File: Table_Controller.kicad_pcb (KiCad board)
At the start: 2 copper layers, 141.6 x 116.3 mm, 98 parts, among them J10 1050171001 Micro Type B, J11 HX JN1.27-2x5 WZ H4.9, J12 Conn_01x04_Pin, J13 Conn_01x14_Pin, J14 2.54 mm header, J15 2.54 mm header, U10 STM32G431K8Tx, U11 LMR380x0, U12 VNH7070, Y10 20 MHz

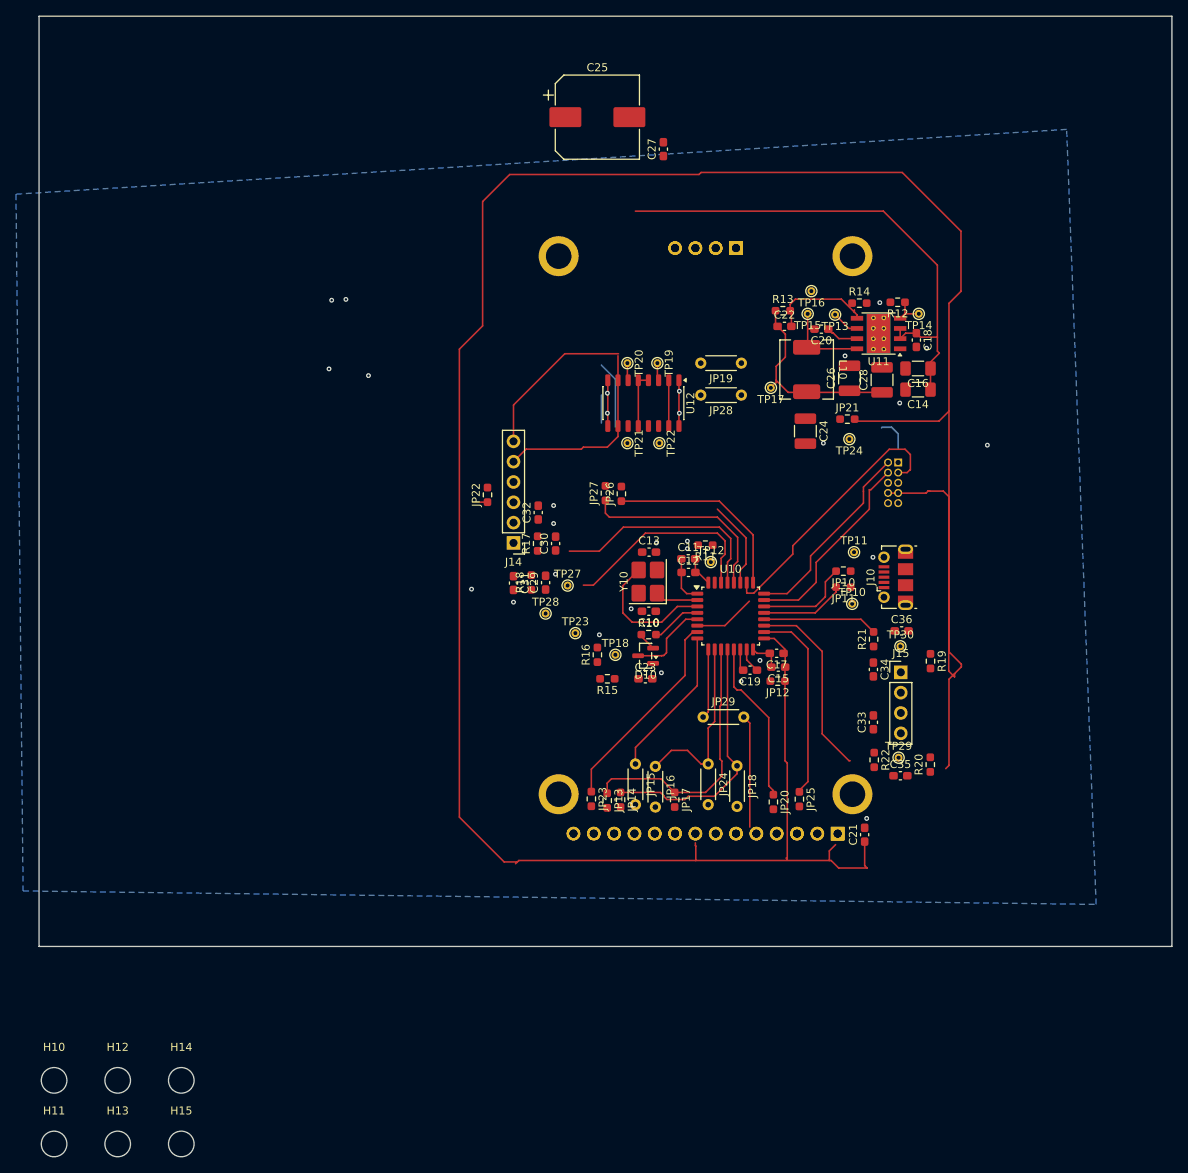
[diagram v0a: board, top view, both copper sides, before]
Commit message: Placement proposal 90%
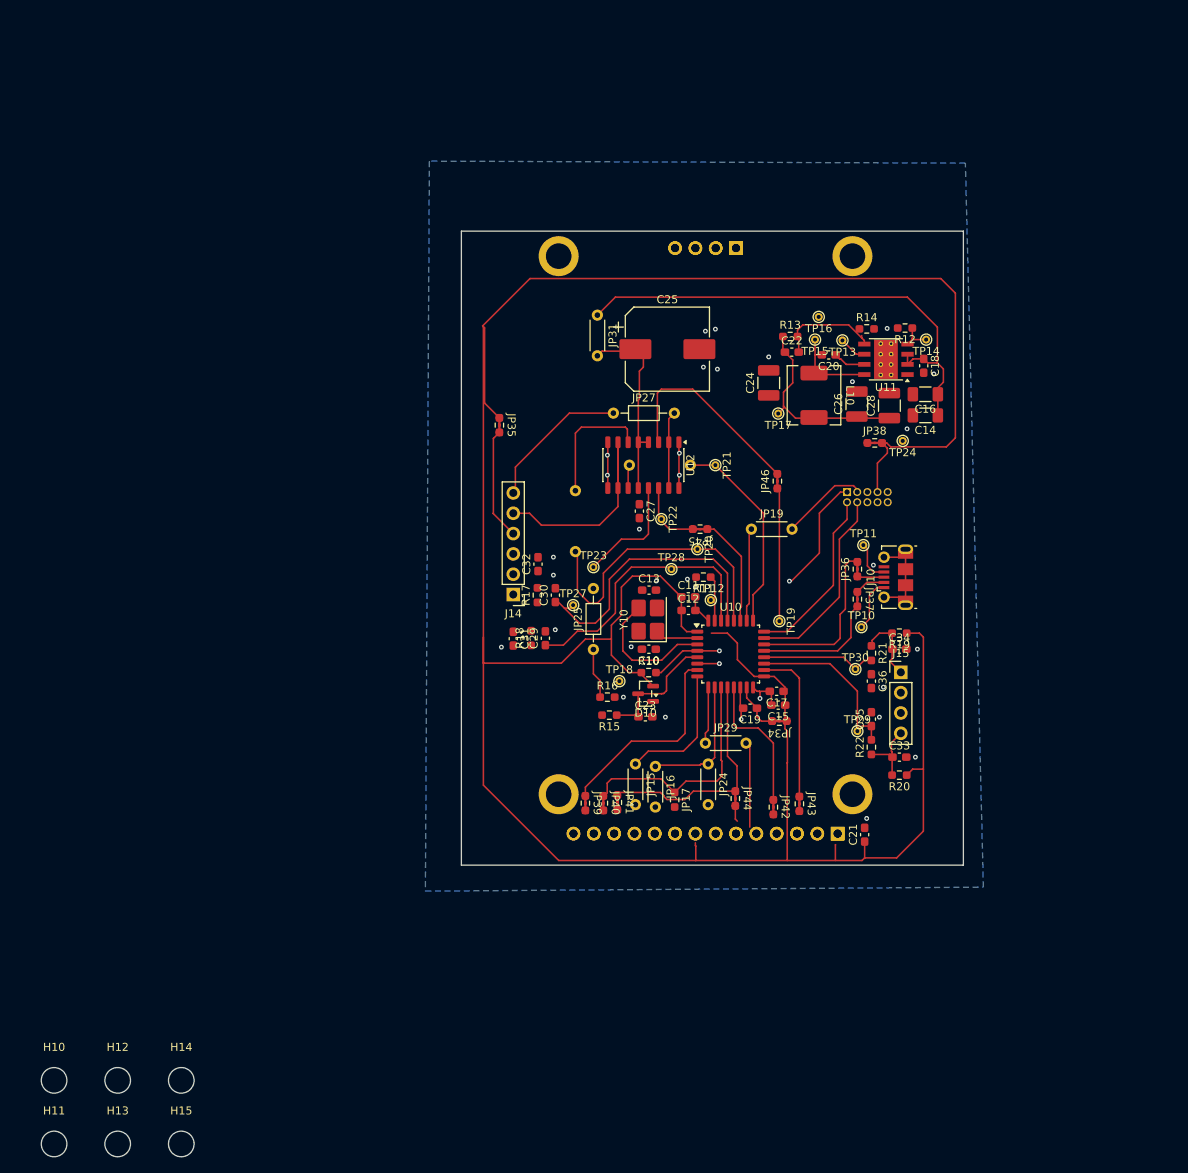
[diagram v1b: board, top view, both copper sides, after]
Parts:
- removed JP10, JP11, JP12, JP13, JP14, JP20, JP21, JP22, JP23: 0R, Resistor_SMD:R_0603_1608Metric_Pad0.98x0.95mm_HandSolder
- removed JP18, JP28: 0R, Resistor_THT:R_Axial_DIN0204_L3.6mm_D1.6mm_P5.08mm_Horizontal
- added JP31: 0R, Resistor_THT:R_Axial_DIN0204_L3.6mm_D1.6mm_P5.08mm_Horizontal, F.Cu at (95.8, 77.5)
- added JP32: 0R, Resistor_THT:R_Axial_DIN0204_L3.6mm_D1.6mm_P7.62mm_Horizontal, B.Cu at (99.8, 96.2)
- added JP34: 0R, Personal:Jumper_0603, F.Cu at (118.5, 128.2)
- added JP35: 0R, Personal:Jumper_0603, F.Cu at (83.5, 91.2)
- added JP36: 0R, Personal:Jumper_0603, F.Cu at (128.2, 109.2)
- added JP37: 0R, Personal:Jumper_0603, F.Cu at (128.2, 113.0)
- added JP38: 0R, Personal:Jumper_0603, F.Cu at (130.4, 93.5)
- added JP39: 0R, Personal:Jumper_0603, F.Cu at (94.2, 138.5)
- added JP40: 0R, Personal:Jumper_0603, F.Cu at (96.5, 138.5)
- added JP41: 0R, Personal:Jumper_0603, F.Cu at (98.2, 138.4)
- added JP42: 0R, Personal:Jumper_0603, F.Cu at (117.8, 139.0)
- added JP43: 0R, Personal:Jumper_0603, F.Cu at (121.0, 138.6)
- added JP44: 0R, Personal:Jumper_0603, F.Cu at (113.0, 137.9)
- added JP45: 0R, Personal:Jumper_0603, F.Cu at (108.6, 104.2)
- added JP46: 0R, Personal:Jumper_0603, F.Cu at (118.2, 98.2)
- JP25, JP27: footprint Resistor_SMD:R_0603_1608Metric_Pad0.98x0.95mm_HandSolder -> Resistor_THT:R_Axial_DIN0204_L3.6mm_D1.6mm_P7.62mm_Horizontal
- JP26: footprint Resistor_SMD:R_0603_1608Metric_Pad0.98x0.95mm_HandSolder -> Resistor_THT:R_Axial_DIN0204_L3.6mm_D1.6mm_P7.62mm_Horizontal; moved to B.Cu
- moved C27 45.3 mm to (101.0, 102.0), turned to -90 degrees
- moved TP19 35.7 mm to (118.5, 115.8)
- moved JP25 31.8 mm to (95.2, 119.3), turned to 90 degrees
- moved C25 30.3 mm to (104.5, 81.8)
- moved TP20 24.8 mm to (108.2, 106.8)
- moved JP19 20.8 mm to (115.0, 104.2), turned to 0 degrees
- moved TP28 16.7 mm to (105.0, 109.2)
- moved TP21 11.3 mm to (110.5, 96.2)
- moved JP27 10.0 mm to (97.8, 89.8), turned to 0 degrees
- moved TP22 9.50 mm to (103.8, 103.0)
- moved TP23 8.55 mm to (95.2, 109.0)
- moved C35 7.95 mm to (130.0, 128.0), turned to 90 degrees
- moved U12 7.75 mm to (101.5, 96.2)
- moved C24 7.57 mm to (117.2, 86.0), turned to 90 degrees
- moved C36 7.33 mm to (130.0, 123.2), turned to -90 degrees
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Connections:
- net Net-(U10-PF0) renamed /XIN
- net Net-(U10-PF1) renamed /XOUT
- C25 pad 1: /S19V5 -> Net-(C25-Pad1)
- C27 pad 1: /S19V5 -> Net-(C25-Pad1)
- J11 pad 3: /SWO -> Net-(J11-Pin_3)
- JP19 pad 1: /SEL0 -> /SWO
- JP19 pad 2: Net-(U12-SEL0) -> Net-(J11-Pin_3)
- JP25 pad 1: /DISP_CS -> Net-(JP25-Pad1)
- JP25 pad 2: Net-(J13-Pin_3) -> Net-(U12-CS)
- JP26 pad 1: /INa -> Net-(U12-INb)
- JP26 pad 2: Net-(U12-INa) -> /INb
- JP27 pad 1: /INb -> /OUTa
- JP27 pad 2: Net-(U12-INb) -> Net-(JP27-Pad2)
- R15 pad 2: Net-(U12-CS) -> Net-(JP25-Pad1)
- R16 pad 1: Net-(U12-CS) -> Net-(JP25-Pad1)
- TP19 pad 1: Net-(U12-INa) -> /INa
- TP20 pad 1: Net-(U12-INb) -> /INb
- TP21 pad 1: Net-(U12-PWM) -> /PWM
- U10 pad 25: /INa -> /PWM
- U10 pad 27: /PWM -> /SEL0
- U10 pad 6: /SEL0 -> /INa
- U12 pad 12: /S19V5 -> Net-(C25-Pad1)
- U12 pad 15: /OUTa -> Net-(JP27-Pad2)
- U12 pad 2: /OUTa -> Net-(JP27-Pad2)
- U12 pad 4: /S19V5 -> Net-(C25-Pad1)
- U12 pad 5: /S19V5 -> Net-(C25-Pad1)
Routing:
- net /NRST: track 10.6 -> 36.2 mm, vias 0 -> 2
- net Net-(C25-Pad1): track 0.00 -> 24.4 mm
- net /SWO: track 33.7 -> 11.7 mm
- net Net-(U12-INa): track 10.7 -> 25.8 mm
- net /PWM: track 11.0 -> 25.6 mm
- net Net-(U12-CS): track 0.00 -> 14.4 mm
- net Net-(J14-Pin_4): track 0.00 -> 14.0 mm
- net /INb: track 25.3 -> 37.3 mm
- net Net-(J10-Shield): track 0.00 -> 11.5 mm
- net Net-(J11-Pin_3): track 0.00 -> 11.0 mm
- net Net-(U12-INb): track 5.68 -> 15.8 mm
- net Net-(JP27-Pad2): track 0.00 -> 9.65 mm
- net /TOP_EOT: track 0.00 -> 9.19 mm
- net /USB_DP: track 11.9 -> 21.0 mm
- net Net-(U12-SEL0): track 0.00 -> 8.78 mm
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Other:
- board size 141.6 x 116.3 mm -> 62.8 x 79.2 mm
- copper layers 2 -> 4

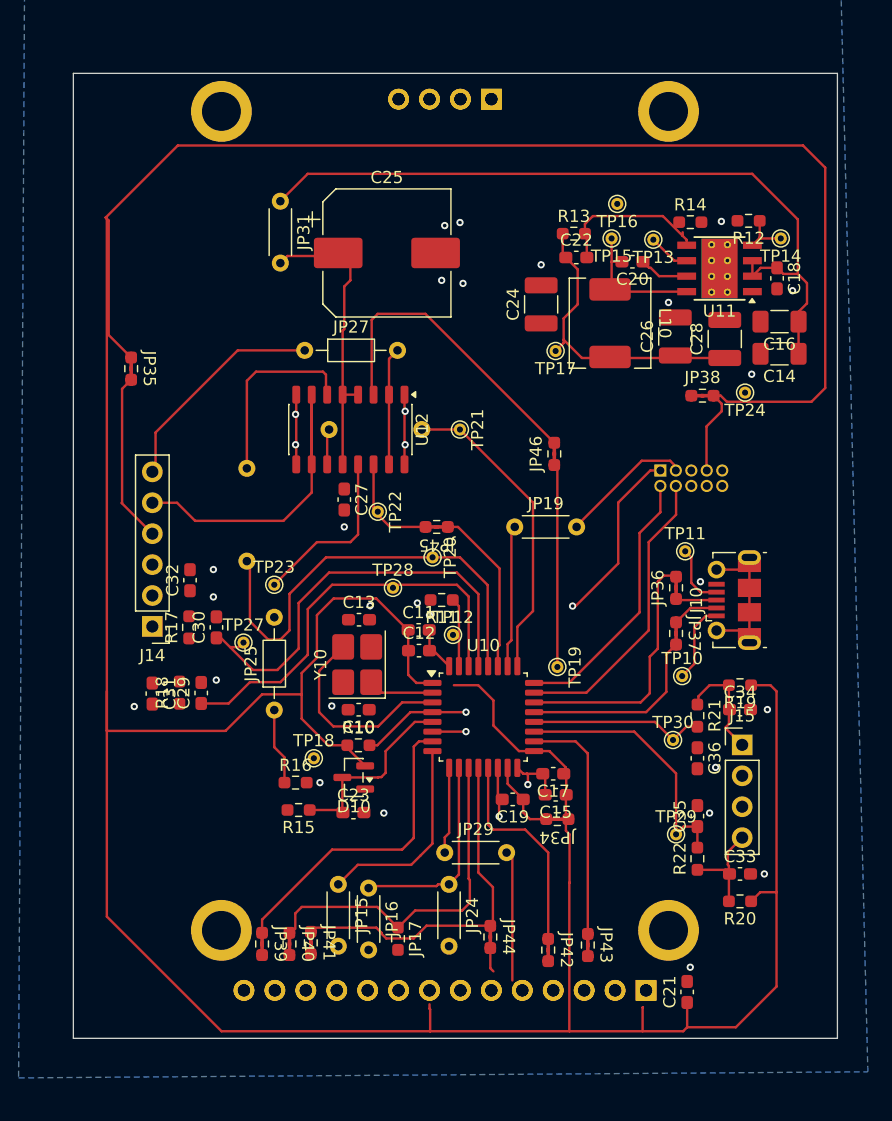
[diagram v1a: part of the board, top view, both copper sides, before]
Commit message: placement 95%
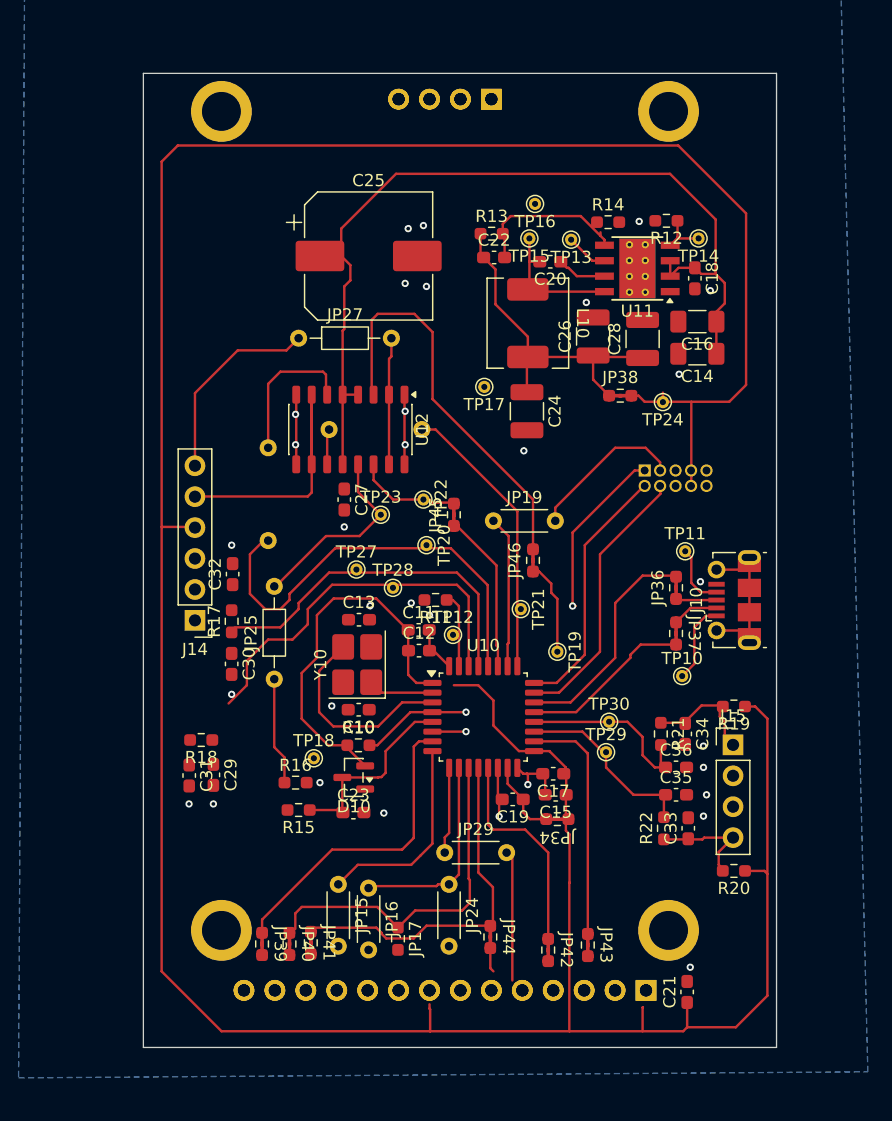
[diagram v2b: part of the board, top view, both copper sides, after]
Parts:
- removed JP31: 0R, Resistor_THT:R_Axial_DIN0204_L3.6mm_D1.6mm_P5.08mm_Horizontal
- removed JP35: 0R, Personal:Jumper_0603
- moved TP21 15.6 mm to (115.5, 111.0)
- moved TP27 11.0 mm to (102.0, 107.8)
- moved TP23 10.5 mm to (104.0, 103.2)
- moved JP46 8.92 mm to (116.5, 107.0)
- moved TP29 8.87 mm to (122.5, 122.8)
- moved C24 8.86 mm to (116.0, 94.8), turned to -90 degrees
- moved C31 7.38 mm to (88.3, 124.7)
- moved C29 6.80 mm to (90.2, 124.6), turned to -90 degrees
- moved TP24 6.79 mm to (127.2, 94.0)
- moved JP38 6.75 mm to (123.7, 93.5)
- moved R12 6.75 mm to (127.5, 79.1)
- moved R14 6.75 mm to (122.7, 79.2)
- moved C14 6.75 mm to (130.0, 90.0)
- moved C16 6.75 mm to (130.0, 87.4)
- moved C18 6.75 mm to (129.8, 83.8)
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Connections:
- C25 pad 1: Net-(C25-Pad1) -> /S19V5
- C27 pad 1: Net-(C25-Pad1) -> /S19V5
- J14 pad 4: Net-(J14-Pin_4) -> /S3V3
- U12 pad 12: Net-(C25-Pad1) -> /S19V5
- U12 pad 4: Net-(C25-Pad1) -> /S19V5
- U12 pad 5: Net-(C25-Pad1) -> /S19V5
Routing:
- net /S3V3: track 349.3 -> 304.7 mm
- net Net-(C25-Pad1): track 24.4 -> 0.00 mm
- net Net-(J14-Pin_4): track 14.0 -> 0.00 mm
- net /S19V5: track 62.1 -> 75.7 mm
- net /INa: track 29.2 -> 20.7 mm
- net Net-(U12-INa): track 25.8 -> 33.3 mm
- net /ENCa_filt: track 36.0 -> 28.8 mm
- net /BOT_filt: track 21.8 -> 15.6 mm
- net /OUTb: track 28.4 -> 23.5 mm
- net Net-(U12-INb): track 15.8 -> 12.2 mm
- net Net-(C22-Pad1): track 24.8 -> 28.0 mm
- net /ENCb_filt: track 34.3 -> 31.8 mm, vias 0 -> 1
- net Net-(JP25-Pad1): track 6.31 -> 8.85 mm
- net /USB_DP: track 21.0 -> 18.6 mm
- net /PWM: track 25.6 -> 23.3 mm
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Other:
- board size 62.8 x 79.2 mm -> 52 x 80 mm
